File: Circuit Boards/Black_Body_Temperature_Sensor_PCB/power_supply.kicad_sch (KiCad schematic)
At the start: 4 parts, among them J3 Barrel_Jack, U5 AMS1117-3.3

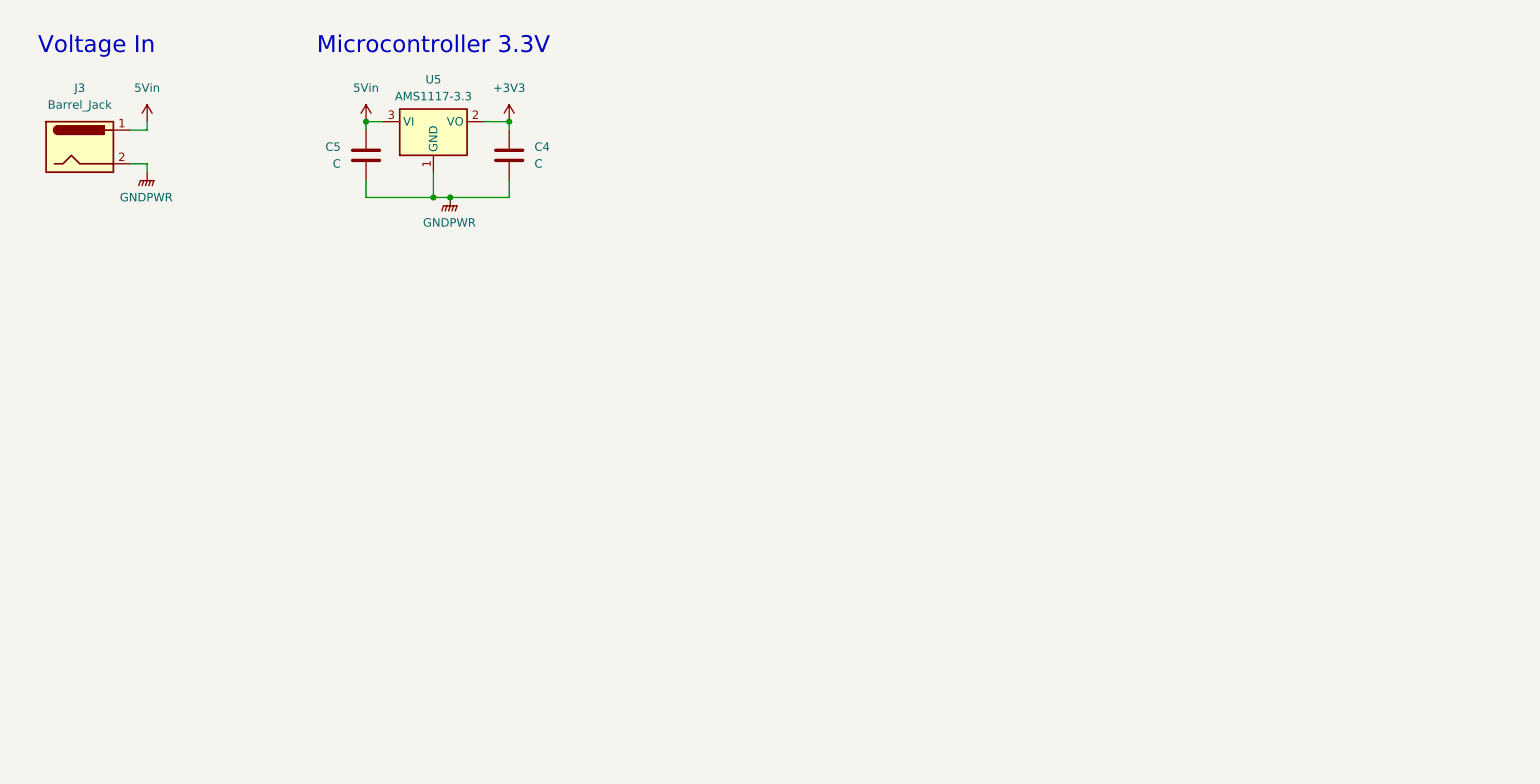
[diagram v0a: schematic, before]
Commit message: Schematic ready for review
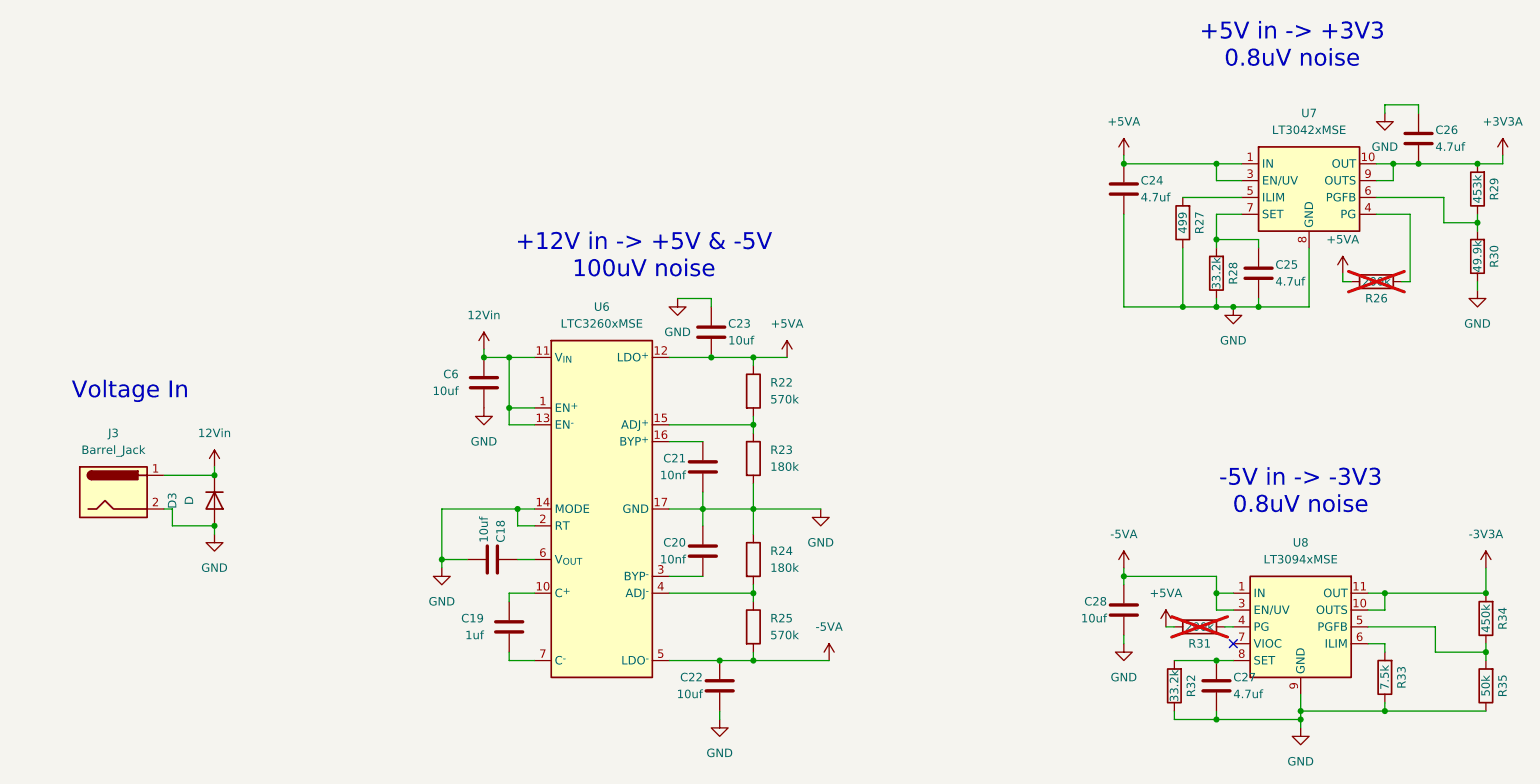
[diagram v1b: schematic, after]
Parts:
- removed C4, C5: C, symbol Device:C
- removed U5: AMS1117-3.3, Package_TO_SOT_SMD:SOT-223-3_TabPin2, symbol Regulator_Linear:AMS1117-3.3
- added C18, C22, C23, C28, C6: 10uf, symbol Device:C
- added C19: 1uf, symbol Device:C
- added C20, C21: 10nf, symbol Device:C
- added C24, C25, C26, C27: 4.7uf, symbol Device:C
- added D3: D, symbol Device:D
- added R22, R25: 570k, symbol Device:R
- added R23, R24: 180k, symbol Device:R
- added R26, R31: 200k, symbol Device:R
- added R27: 499, symbol Device:R
- added R28, R32: 33.2k, symbol Device:R
- added R29: 453k, symbol Device:R
- added R30: 49.9k, symbol Device:R
- added R33: 7.5k, symbol Device:R
- added R34: 450k, symbol Device:R
- added R35: 50k, symbol Device:R
- added U6: LTC3260xMSE, Package_SO:MSOP-16-1EP_3x4.039mm_P0.5mm_EP1.651x2.845mm, symbol Regulator_SwitchedCapacitor:LTC3260xMSE
- added U7: LT3042xMSE, Package_SO:MSOP-10-1EP_3x3mm_P0.5mm_EP1.68x1.88mm, symbol Regulator_Linear:LT3042xMSE
- added U8: LT3094xMSE, Package_SO:MSOP-12-1EP_3x4.039mm_P0.65mm_EP1.651x2.845mm, symbol Regulator_Linear:LT3094xMSE
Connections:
- net 5Vin renamed 12Vin
- net 12Vin: now also C6.1, D3.1 (K), U6.1 (EN^{+}), U6.11 (V_{IN}), U6.13 (EN^{-})
- net GNDPWR renamed GND
- net GND: now also C18.2, C20.1, C21.2, C22.2, C23.1, C24.2, C25.2, C26.1, C27.2, C28.2, C6.2, D3.2 (A), R23.2, R24.1, R27.1, R28.1, R30.1, R32.1, R33.1, R35.1, U6.14 (MODE), U6.17 (GND), U6.2 (RT), U7.11 (GND), U7.8 (GND), U8.9 (GND)
- new net: C21.1, U6.16 (BYP^{+})
- new net: C18.1, U6.6 (V_{OUT})
- new net: R24.2, R25.1, U6.4 (ADJ^{-})
- new net: R31.1, U8.4 (PG)
- new net: R34.1, R35.2, U8.5 (PGFB)
- new net: R33.2, U8.6 (ILIM)
- new net: C27.1, R32.2, U8.8 (SET)
- new net: R29.1, R30.2, U7.6 (PGFB)
- new net: R26.1, U7.4 (PG)
- new net: R27.2, U7.5 (ILIM)
- new net: C25.1, R28.2, U7.7 (SET)
- new net: R22.2, R23.1, U6.15 (ADJ^{+})
- new net: C19.1, U6.10 (C^{+})
- new net: C20.2, U6.3 (BYP^{-})
- new net: C19.2, U6.7 (C^{-})
- new net +3V3A: C26.2, R29.2, U7.10 (OUT), U7.9 (OUTS)
- new net +5VA: C23.2, C24.1, R22.1, R26.2, R31.2, U6.12 (LDO^{+}), U7.1 (IN), U7.2 (IN), U7.3 (EN/UV)
- new net -3V3A: R34.2, U8.10 (OUTS), U8.11 (OUT), U8.12 (OUT)
- new net -5VA: C22.1, C28.1, R25.2, U6.5 (LDO^{-}), U8.1 (IN), U8.13 (IN), U8.2 (IN), U8.3 (EN/UV)
- no-connect marks 0 -> 1
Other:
- note added: "+12V in -> +5V & -5V 100uV noise"
- note added: "+5V in -> +3V3 0.8uV noise"
- note added: "-5V in -> -3V3 0.8uV noise"
- note removed: "Microcontroller 3.3V"
- moved on the sheet: J3
